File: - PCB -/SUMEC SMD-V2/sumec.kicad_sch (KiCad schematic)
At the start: 2 parts

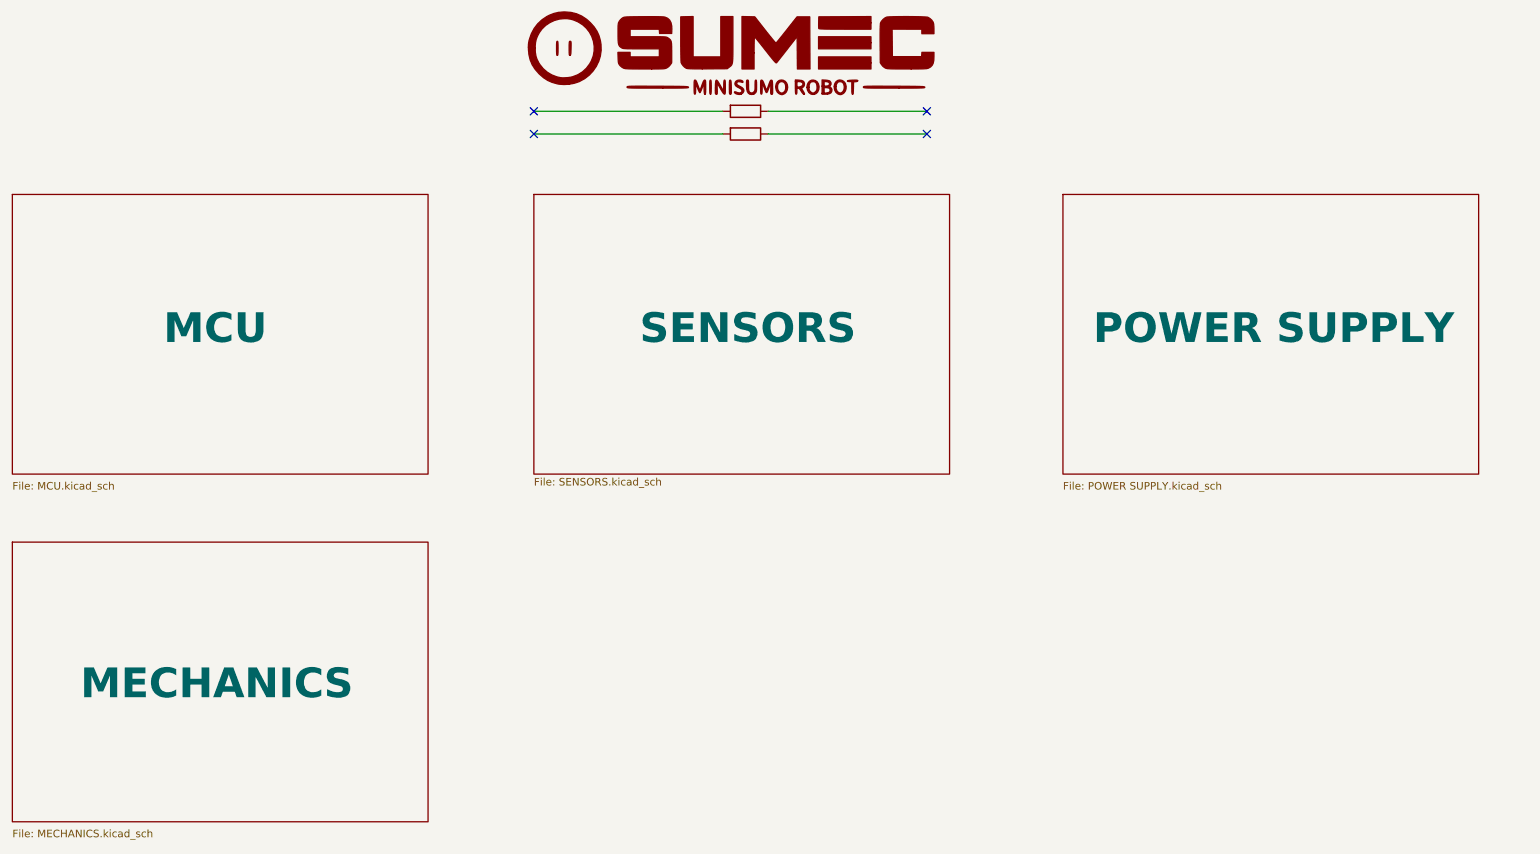
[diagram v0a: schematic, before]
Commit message: mateji co jsi kurva delal v slozce PCB??
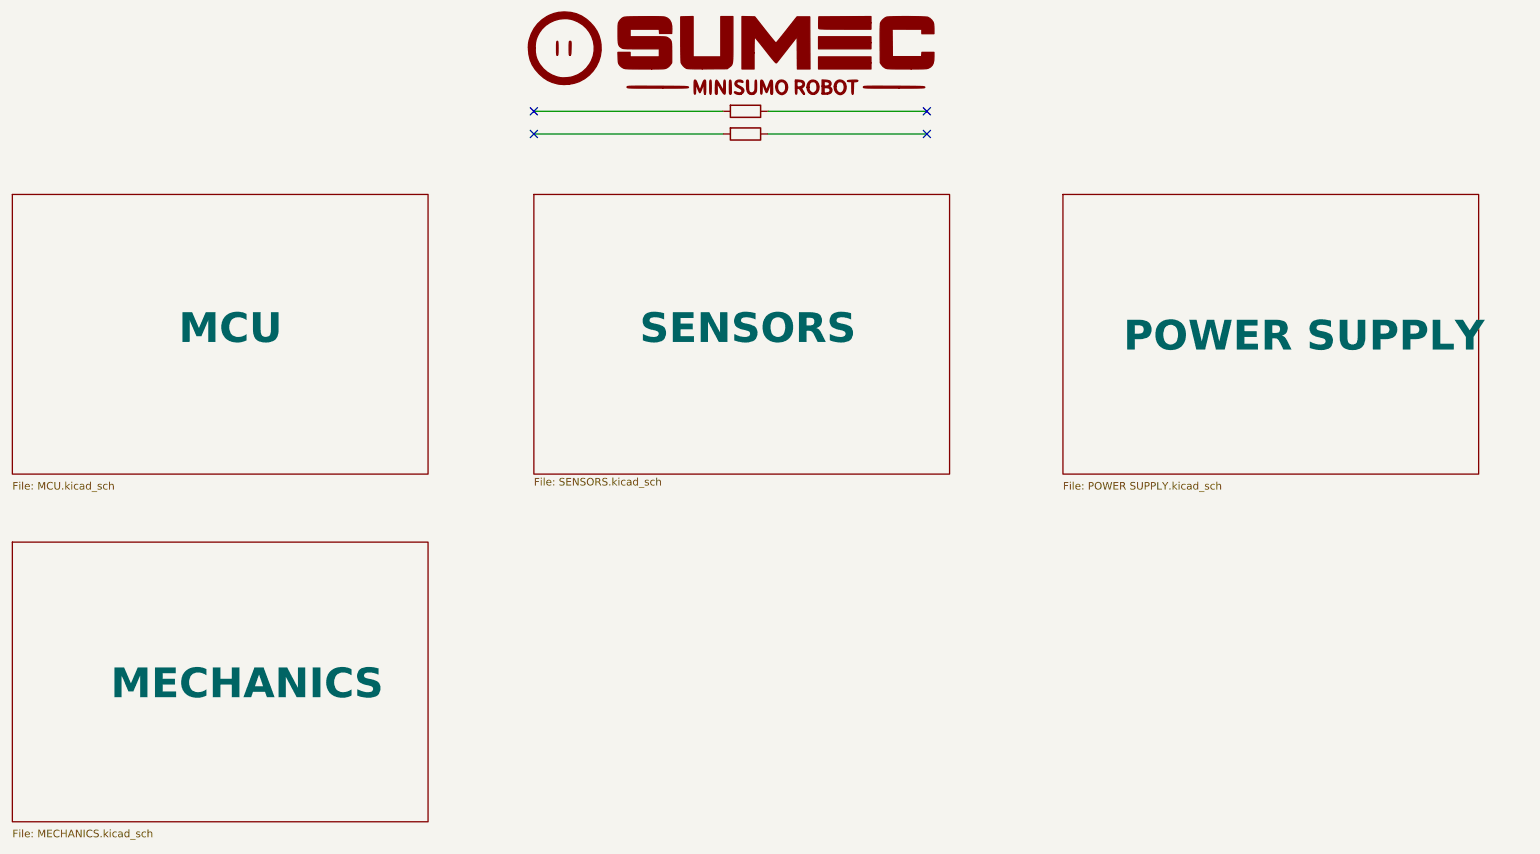
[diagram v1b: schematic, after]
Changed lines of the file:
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@@
     (in_bom yes) (on_board yes) (dnp no) (fields_autoplaced)
     (property "Reference" "R3" (at 151.13 39.37 90)
-      (effects (font (size 1.27 1.27)) hide)
+      (effects (font (face "Bahnschrift") (size 1.27 1.27)) hide)
     )
     (property "Value" "R" (at 151.13 36.83 90)
-      (effects (font (size 1.27 1.27)) hide)
+      (effects (font (face "Bahnschrift") (size 1.27 1.27)) hide)
     )
     (property "Footprint" "sumec-smdV2_library:R2D2" (at 151.13 32.512 90)
-      (effects (font (size 1.27 1.27)) hide)
+      (effects (font (face "Bahnschrift") (size 1.27 1.27)) hide)
     )
     (property "Datasheet" "~" (at 151.13 34.29 0)
-      (effects (font (size 1.27 1.27)) hide)
+      (effects (font (face "Bahnschrift") (size 1.27 1.27)) hide)
     )
     (pin "1")
@@
     (in_bom yes) (on_board yes) (dnp no) (fields_autoplaced)
     (property "Reference" "R8" (at 151.13 43.18 90)
-      (effects (font (size 1.27 1.27)) hide)
+      (effects (font (face "Bahnschrift") (size 1.27 1.27)) hide)
     )
     (property "Value" "R" (at 151.13 40.64 90)
-      (effects (font (size 1.27 1.27)) hide)
+      (effects (font (face "Bahnschrift") (size 1.27 1.27)) hide)
     )
     (property "Footprint" "sumec-smdV2_library:Logo" (at 151.13 36.322 90)
-      (effects (font (size 1.27 1.27)) hide)
+      (effects (font (face "Bahnschrift") (size 1.27 1.27)) hide)
     )
     (property "Datasheet" "~" (at 151.13 38.1 0)
-      (effects (font (size 1.27 1.27)) hide)
+      (effects (font (face "Bahnschrift") (size 1.27 1.27)) hide)
     )
     (pin "1")
@@
     (in_bom yes) (on_board yes) (dnp no) (fields_autoplaced)
     (property "Reference" "#G1" (at 147.32 14.7743 0)
-      (effects (font (size 1.27 1.27)) hide)
+      (effects (font (face "Bahnschrift") (size 1.27 1.27)) hide)
     )
     (property "Value" "LOGO" (at 147.32 36.0257 0)
-      (effects (font (size 1.27 1.27)) hide)
+      (effects (font (face "Bahnschrift") (size 1.27 1.27)) hide)
     )
     (property "Footprint" "" (at 147.32 25.4 0)
-      (effects (font (size 1.27 1.27)) hide)
+      (effects (font (face "Bahnschrift") (size 1.27 1.27)) hide)
     )
     (property "Datasheet" "" (at 147.32 25.4 0)
-      (effects (font (size 1.27 1.27)) hide)
+      (effects (font (face "Bahnschrift") (size 1.27 1.27)) hide)
     )
     (instances
@@
     (stroke (width 0.1524) (type solid) (color 0 0 0 1))
     (fill (color 255 255 255 1.0000))
-    (property "Sheetname" "MECHANICS" (at 39.37 133.35 0)
-      (effects (font (size 5 5) bold (color 0 0 0 1)) (justify left bottom))
+    (property "Sheetname" "MECHANICS" (at 44.45 133.35 0)
+      (effects (font (face "Bahnschrift") (size 5 5) bold (color 0 0 0 1)) (justify left bottom))
     )
     (property "Sheetfile" "MECHANICS.kicad_sch" (at 27.94 154.94 0)
-      (effects (font (size 1.27 1.27) (color 0 0 0 1)) (justify left top))
+      (effects (font (face "Bahnschrift") (size 1.27 1.27) (color 0 0 0 1)) (justify left top))
     )
     (instances
@@
     (stroke (width 0.1524) (type solid) (color 0 0 0 1))
     (fill (color 255 255 255 1.0000))
-    (property "Sheetname" "MCU" (at 53.34 73.66 0)
-      (effects (font (size 5 5) bold (color 0 0 0 1)) (justify left bottom))
+    (property "Sheetname" "MCU" (at 55.88 73.66 0)
+      (effects (font (face "Bahnschrift") (size 5 5) bold (color 0 0 0 1)) (justify left bottom))
     )
     (property "Sheetfile" "MCU.kicad_sch" (at 27.94 96.52 0)
-      (effects (font (size 1.27 1.27) (color 0 0 0 1)) (justify left top))
+      (effects (font (face "Bahnschrift") (size 1.27 1.27) (color 0 0 0 1)) (justify left top))
     )
     (instances
@@
     (stroke (width 0.1524) (type solid) (color 0 0 0 1))
     (fill (color 255 255 255 1.0000))
-    (property "Sheetname" "POWER SUPPLY" (at 209.55 73.66 0)
-      (effects (font (size 5 5) bold (color 0 0 0 1)) (justify left bottom))
+    (property "Sheetname" "POWER SUPPLY" (at 214.63 74.93 0)
+      (effects (font (face "Bahnschrift") (size 5 5) bold (color 0 0 0 1)) (justify left bottom))
     )
     (property "Sheetfile" "POWER SUPPLY.kicad_sch" (at 204.47 96.52 0)
-      (effects (font (size 1.27 1.27) (color 0 0 0 1)) (justify left top))
+      (effects (font (face "Bahnschrift") (size 1.27 1.27) (color 0 0 0 1)) (justify left top))
     )
     (instances
@@
     (fill (color 255 255 255 1.0000))
     (property "Sheetname" "SENSORS" (at 133.35 73.66 0)
-      (effects (font (size 5 5) bold (color 0 0 0 1)) (justify left bottom))
+      (effects (font (face "Bahnschrift") (size 5 5) bold (color 0 0 0 1)) (justify left bottom))
     )
     (property "Sheetfile" "SENSORS.kicad_sch" (at 115.57 95.8346 0)
-      (effects (font (size 1.27 1.27) (color 0 0 0 1)) (justify left top))
+      (effects (font (face "Bahnschrift") (size 1.27 1.27) (color 0 0 0 1)) (justify left top))
     )
     (property "Field2" "" (at 115.57 48.26 0)
-      (effects (font (size 1.27 1.27)) hide)
+      (effects (font (face "Bahnschrift") (size 1.27 1.27)) hide)
     )
     (instances
